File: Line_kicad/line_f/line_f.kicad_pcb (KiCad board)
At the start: 2 copper layers, 137.5 x 159.5 mm, 15 parts, among them M2 Motor_DC, M3 Motor_DC, SW1 SW_SPST, SW2 SW_SPDT, SW3 SW_Push, SW4 SW_Push, U1 TB6612FNG_LINE, m1 BLACKPILL

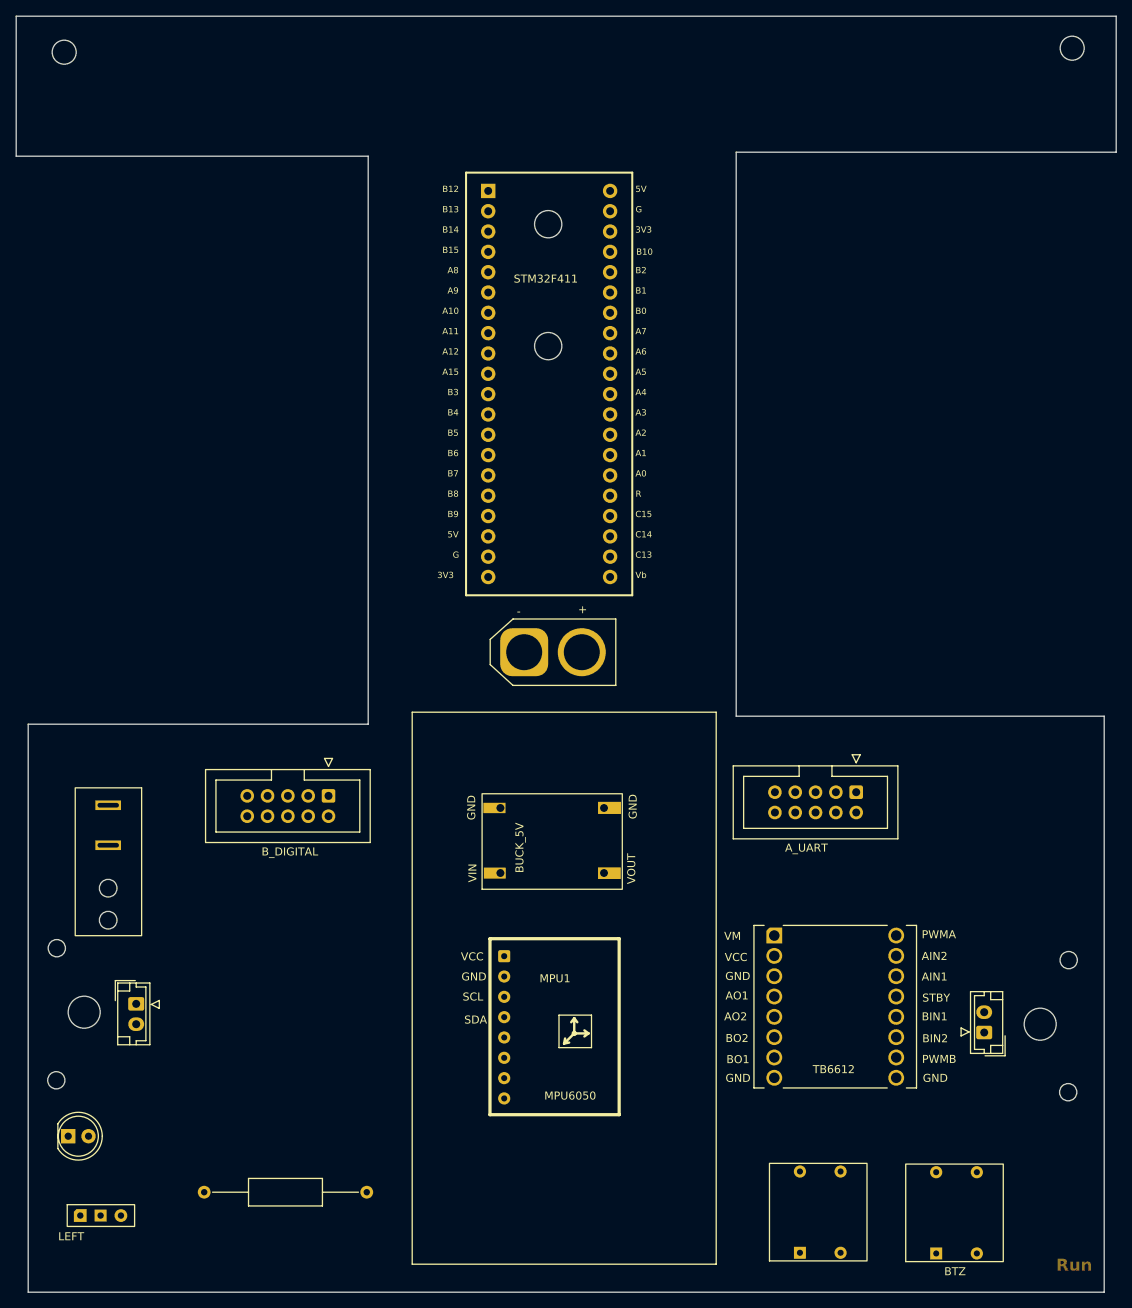
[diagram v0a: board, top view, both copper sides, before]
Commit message: 4#
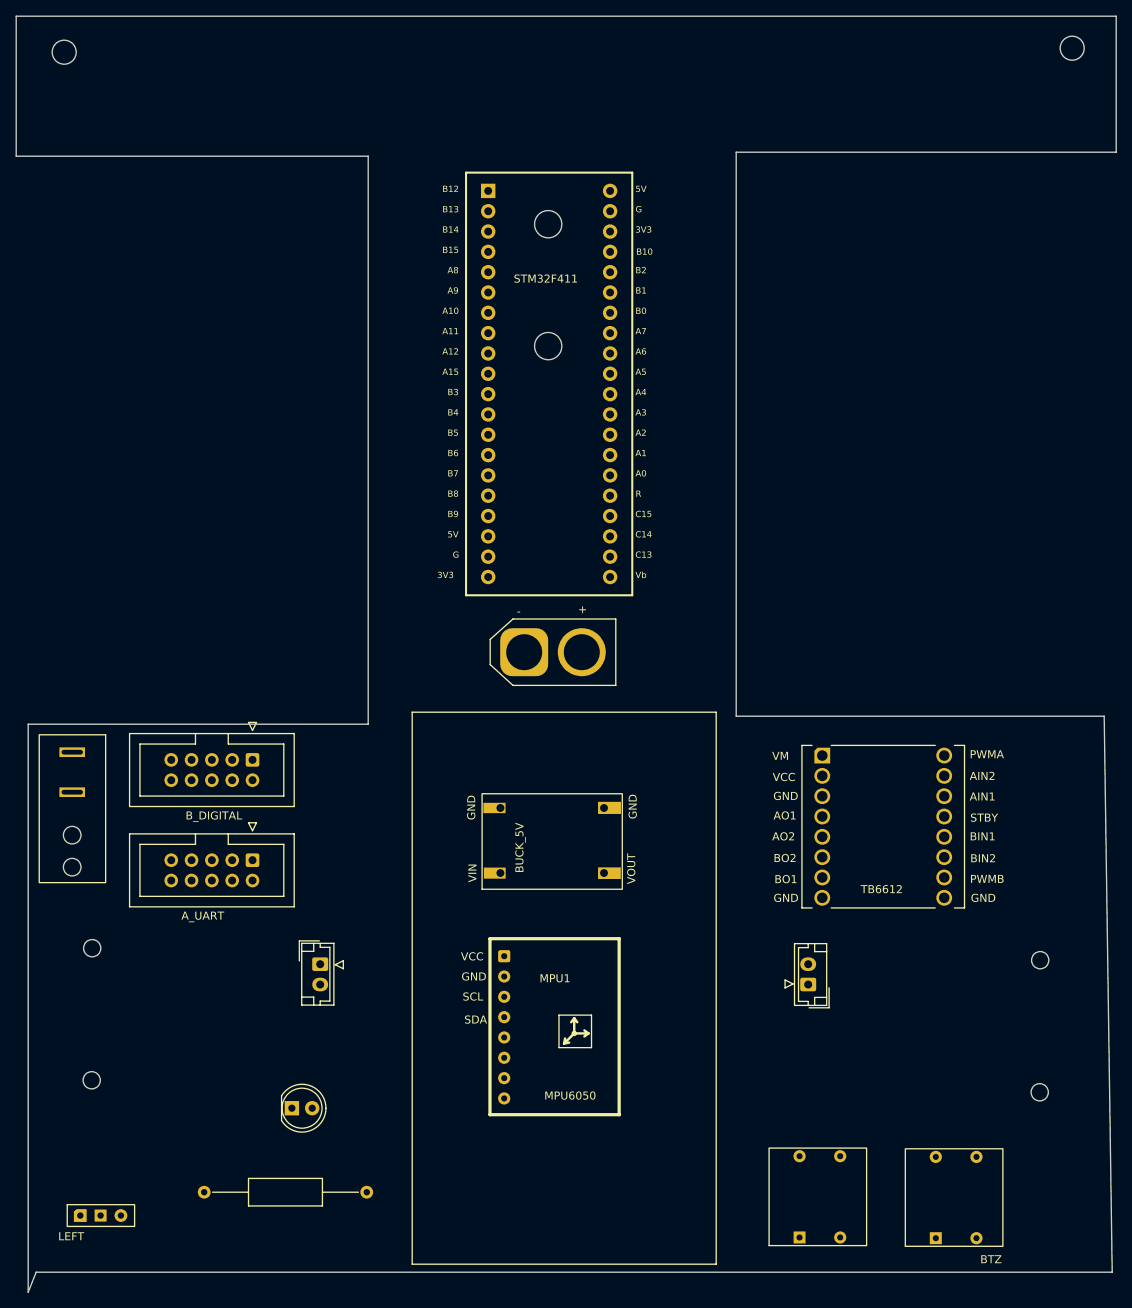
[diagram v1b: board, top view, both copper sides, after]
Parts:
- moved LSA_UART1 75.9 mm to (60.7, 138.1)
- moved D1 28.2 mm to (59.9, 167.8)
- moved M3 23.5 mm to (57.5, 146.4)
- moved U1 23.3 mm to (132.4, 127.8)
- moved M2 22.8 mm to (127.5, 146.2)
- moved LSA_DIGITAL1 10.5 mm to (63.1, 122.6)
- moved SW1 8.01 mm to (31.0, 125.7)
- moved SW3 1.91 mm to (124.0, 174.6)
- moved SW4 1.91 mm to (141.0, 174.7)
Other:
- outline, holes or cut-outs redrawn
- board text removed: "Run"
- board text removed: "Run2'"
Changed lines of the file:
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@@
 	(footprint "LINE_F_FOOT_LIB:LED_LINE"
 		(layer "F.Cu")
-		(at 31.95 171.31)
+		(at 59.91 167.81)
 		(property "Reference" "D1"
 			(at -3 -6 0)
@@
 	(footprint "LINE_F_FOOT_LIB:LSA_UART"
 		(layer "F.Cu")
-		(at 136.2 129.59)
+		(at 60.74 138.09)
 		(property "Reference" "LSA_UART1"
 			(at 1.2625 -0.91 0)
@@
 	(footprint "LINE_F_FOOT_LIB:connector_motor"
 		(layer "F.Cu")
-		(at 149.48 152.18 90)
+		(at 127.48 146.18 90)
 		(property "Reference" "M2"
 			(at 0 -0.5 90)
@@
 	(footprint "LINE_F_FOOT_LIB:push_button"
 		(layer "F.Cu")
-		(at 124 176.5 90)
+		(at 123.952 174.588 90)
 		(property "Reference" "SW3"
 			(at 0.762 -3.302 90)
@@
 	(footprint "LINE_F_FOOT_LIB:battery_sw"
 		(layer "F.Cu")
-		(at 35.5 132.315 -90)
+		(at 31 125.685 -90)
 		(property "Reference" "SW1"
 			(at 0.06 5.17 90)
@@
 	(footprint "LINE_F_FOOT_LIB:push_button"
 		(layer "F.Cu")
-		(at 141.032 176.588 90)
+		(at 140.984 174.676 90)
 		(property "Reference" "SW4"
 			(at 0.762 -3.302 90)
@@
 	(footprint "LINE_F_FOOT_LIB:LSA_DIGITAL"
 		(layer "F.Cu")
-		(at 72.6 127.11)
+		(at 63.1 122.61)
 		(property "Reference" "LSA_DIGITAL1"
 			(at 0 -0.5 0)
@@
 	(footprint "LINE_F_FOOT_LIB:TB6612FNG_LINE"
 		(layer "F.Cu")
-		(at 126.38 150.31)
+		(at 132.38 127.81)
 		(property "Reference" "U1"
 			(at 0.17 -8.12 0)
@@
 	(footprint "LINE_F_FOOT_LIB:connector_motor"
 		(layer "F.Cu")
-		(at 34.52 151.32 -90)
+		(at 57.52 146.36 -90)
 		(property "Reference" "M3"
 			(at 0 -0.5 -90)
@@
 	(gr_poly
 		(pts
-			(xy 25.5 186) (xy 160 186) (xy 160 114) (xy 114 114) (xy 114 43.5) (xy 161.5 43.5) (xy 161.5 26.5)
+			(xy 26.5 183.5) (xy 161 183.5) (xy 160 114) (xy 114 114) (xy 114 43.5) (xy 161.5 43.5) (xy 161.5 26.5)
 			(xy 24 26.5) (xy 24 44) (xy 68 44) (xy 68 115) (xy 25.5 115) (xy 25.5 186)
 		)
@@
 	)
 	(gr_circle
-		(center 152 152.5)
-		(end 154 152.5)
-		(stroke
-			(width 0.05)
-			(type default)
-		)
-		(fill none)
-		(layer "Edge.Cuts")
-	)
-	(gr_circle
-		(center 155.5 161)
-		(end 156.262 161.762)
+		(center 151.93837 161.01)
+		(end 152.70037 161.772)
 		(stroke
 			(width 0.05)
@@
 	)
 	(gr_circle
-		(center 32.5 151)
-		(end 34.5 151)
-		(stroke
-			(width 0.05)
-			(type default)
-		)
-		(fill none)
-		(layer "Edge.Cuts")
-	)
-	(gr_circle
-		(center 29.016 159.51)
-		(end 29.778 160.272)
+		(center 33.43837 159.51)
+		(end 34.20037 160.272)
 		(stroke
 			(width 0.05)
@@
 	)
 	(gr_circle
-		(center 29.07763 143)
-		(end 29.83963 143.762)
+		(center 152 144.5)
+		(end 152.762 145.262)
 		(stroke
 			(width 0.05)
@@
 	)
 	(gr_circle
-		(center 155.56163 144.49)
-		(end 156.32363 145.252)
+		(center 33.5 143)
+		(end 34.262 143.762)
 		(stroke
 			(width 0.05)
@@
 		(layer "Edge.Cuts")
 	)
-	(gr_text "Run"
-		(at 154 183.5 0)
-		(layer "F.Cu")
-		(effects
-			(font
-				(size 1.5 1.5)
-				(thickness 0.3)
-				(bold yes)
-			)
-			(justify left bottom)
-		)
-	)
 	(gr_text "BTZ"
-		(at 140 184 0)
+		(at 144.5 182.5 0)
 		(layer "F.SilkS")
 		(effects
@@
 		)
 	)
-	(gr_text "Run2'"
-		(at 154.5 180 0)
-		(layer "F.Mask")
-		(effects
-			(font
-				(size 1 1)
-				(thickness 0.15)
+	(dimension
+		(type aligned)
+		(layer "F.Cu")
+		(pts
+			(xy 48.5 151) (xy 25.5 151)
+		)
+		(height 0)
+		(gr_text "23.0000 mm"
+			(at 37 149.2 0)
+			(layer "F.Cu")
+			(effects
+				(font
+					(size 1.5 1.5)
+					(thickness 0.3)
+				)
 			)
-			(justify left bottom)
 		)
+		(format
+			(prefix "")
+			(suffix "")
+			(units 3)
+			(units_format 1)
+			(precision 4)
+		)
+		(style
+			(thickness 0.2)
+			(arrow_length 1.27)
+			(text_position_mode 0)
+			(extension_height 0.58642)
+			(extension_offset 0.5) keep_text_aligned)
+	)
+	(dimension
+		(type aligned)
+		(layer "F.Cu")
+		(pts
+			(xy 160 152) (xy 137 152)
+		)
+		(height 0)
+		(gr_text "23.0000 mm"
+			(at 148.5 150.2 0)
+			(layer "F.Cu")
+			(effects
+				(font
+					(size 1.5 1.5)
+					(thickness 0.3)
+				)
+			)
+		)
+		(format
+			(prefix "")
+			(suffix "")
+			(units 3)
+			(units_format 1)
+			(precision 4)
+		)
+		(style
+			(thickness 0.2)
+			(arrow_length 1.27)
+			(text_position_mode 0)
+			(extension_height 0.58642)
+			(extension_offset 0.5) keep_text_aligned)
 	)
 	(group ""
